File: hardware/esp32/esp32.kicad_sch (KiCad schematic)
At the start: 15 parts, among them J1 Conn_01x02, J2 Conn_01x02, J3 Conn_01x02, J4 Conn_01x02, J5 Conn_01x02, U2 ESP32-S3-MINI-1-N8

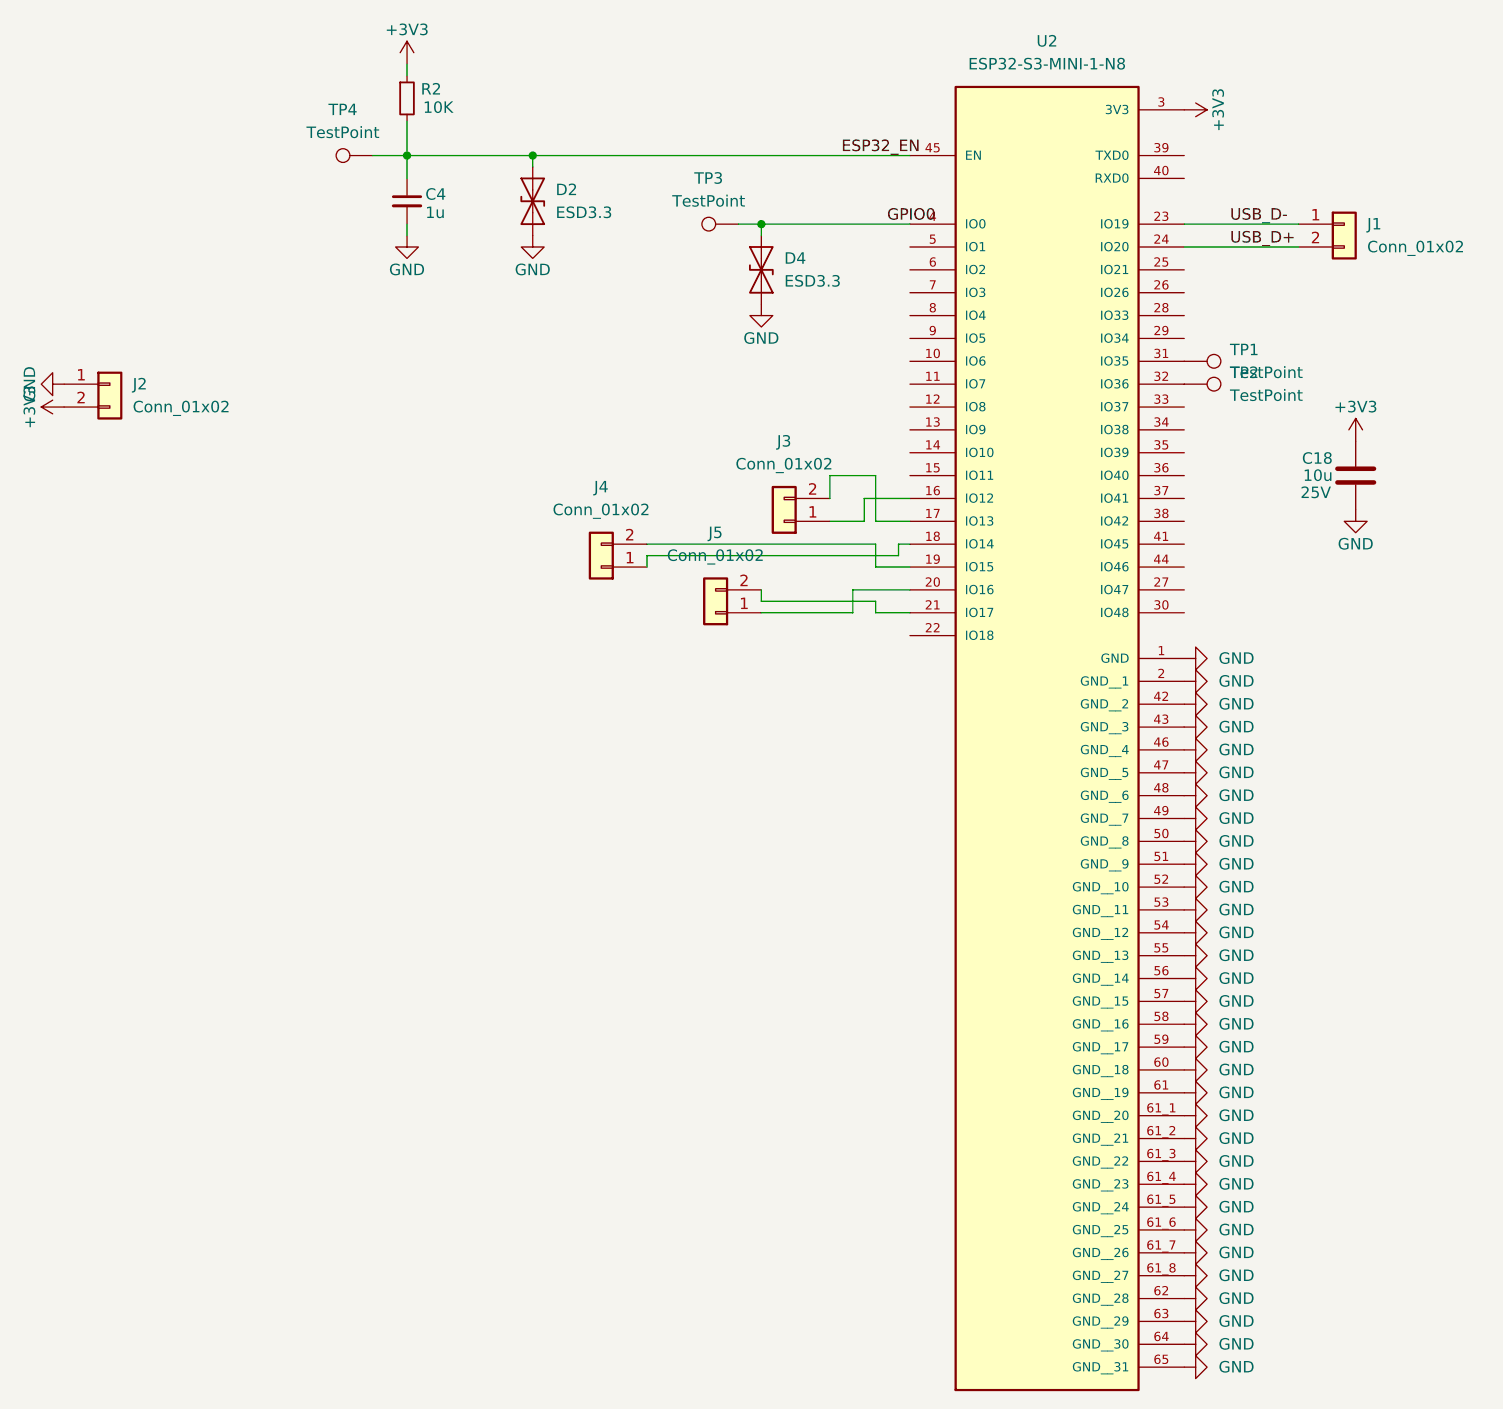
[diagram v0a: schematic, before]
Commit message: esp32 routing
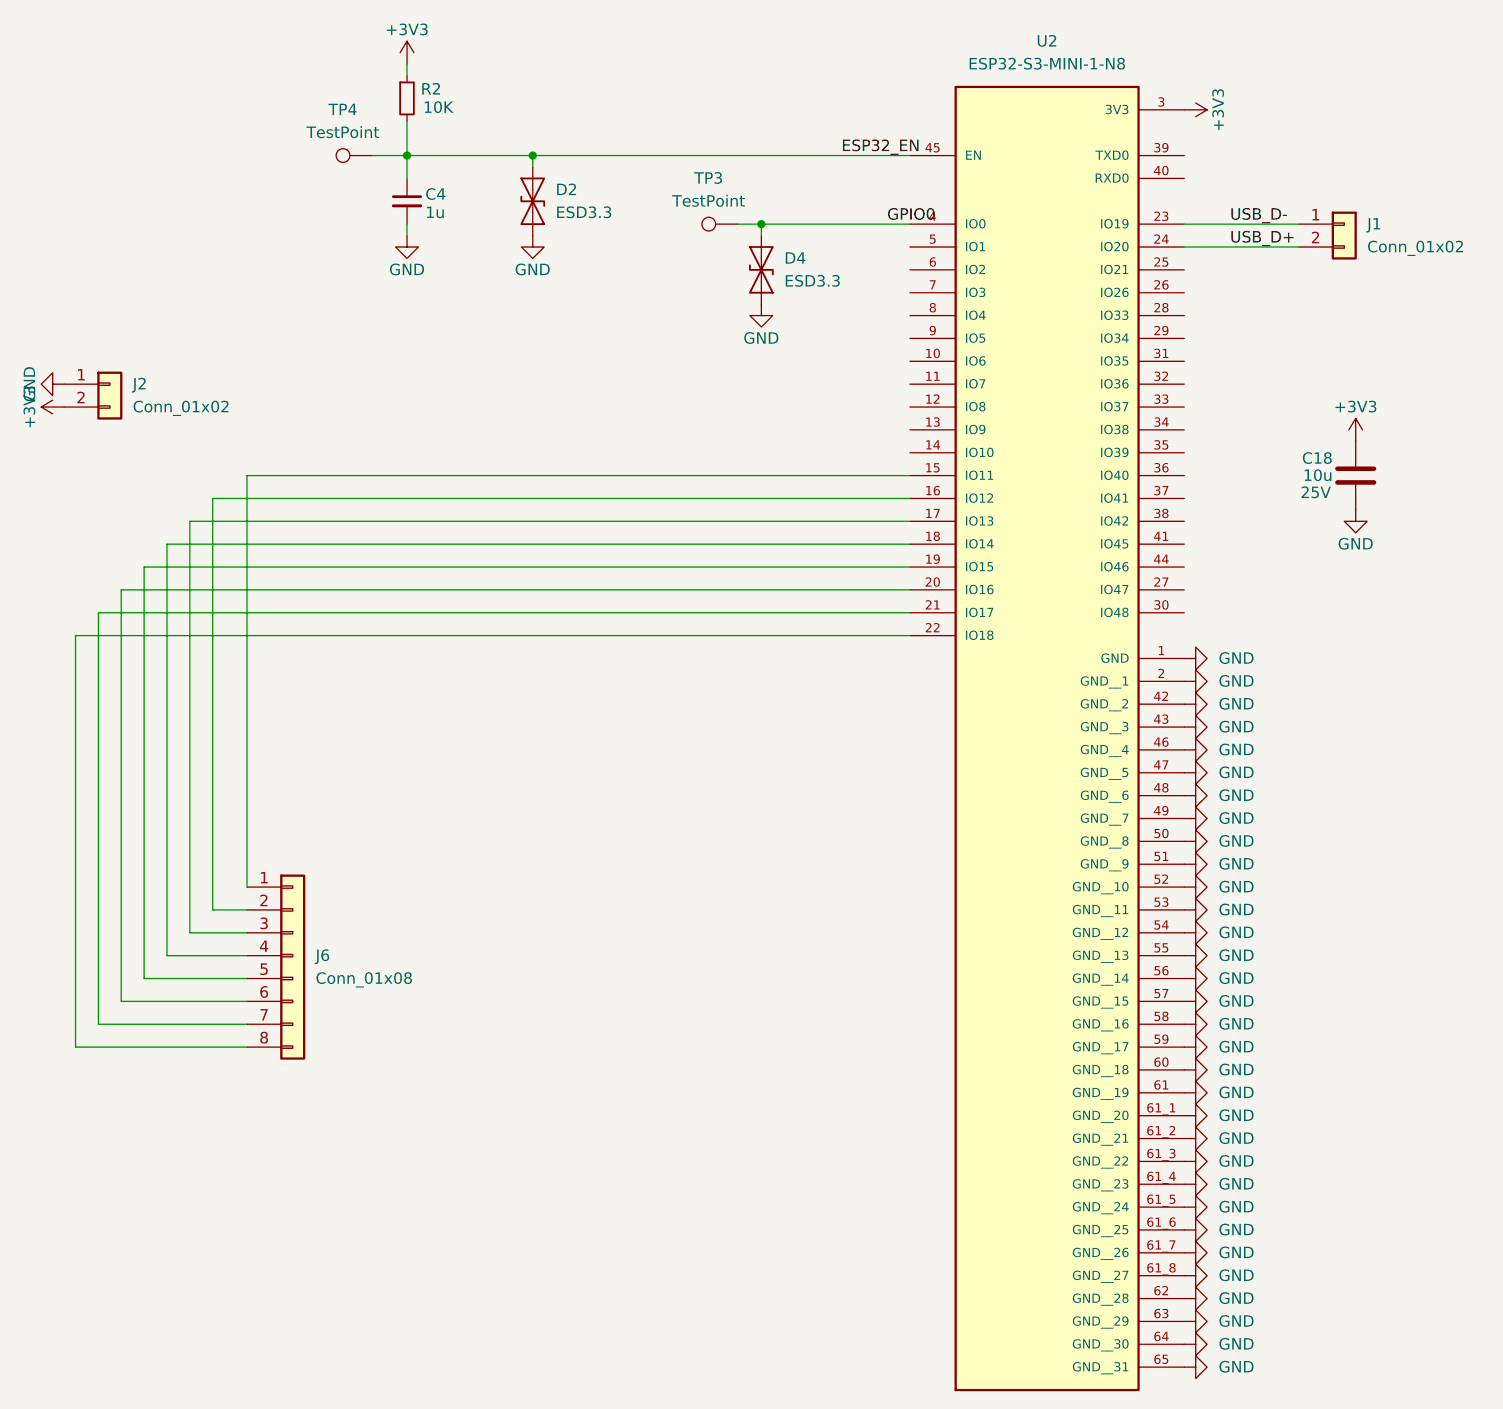
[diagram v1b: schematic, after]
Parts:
- removed J3, J4, J5: Conn_01x02, Connector_JST:JST_SHL_SM02B-SHLS-TF_1x02-1MP_P1.00mm_Horizontal, symbol Connector_Generic:Conn_01x02
- removed TP1, TP2: TestPoint, TestPoint:TestPoint_Pad_1.0x1.0mm, symbol Connector:TestPoint
- added J6: Conn_01x08, Connector_JST:JST_SHL_SM08B-SHLS-TF_1x08-1MP_P1.00mm_Horizontal, symbol Connector_Generic:Conn_01x08
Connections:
- net at U2.15 (IO11): now also J6.1 (Pin_1)
- net at U2.16 (IO12): now also J6.2 (Pin_2)
- net at U2.17 (IO13): now also J6.3 (Pin_3)
- net at U2.18 (IO14): now also J6.4 (Pin_4)
- net at U2.19 (IO15): now also J6.5 (Pin_5)
- net at U2.20 (IO16): now also J6.6 (Pin_6)
- net at U2.21 (IO17): now also J6.7 (Pin_7)
- net at U2.22 (IO18): now also J6.8 (Pin_8)
